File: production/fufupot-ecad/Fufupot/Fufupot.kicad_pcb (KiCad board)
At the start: 4 copper layers, 127 x 127 mm, 56 parts, among them IC1 FOD3150, J1 Conn_01x04, J10 Conn_01x03, J11 Conn_01x03, J12 Conn_01x02, J2 USB_B, J3 Conn_01x03, J4 Conn_01x02, J5 Conn_01x02, J6 Conn_01x02, J7 Conn_01x02, J8 Conn_01x04, J9 Conn_01x02, SW1 SW_Push, SW2 SW_Push, U1 USBLC6-2SC6, U2 LM5165DRC, U3 FT232RL, U4 ATMEGA328P-PN, U5 STGP8NC60KD

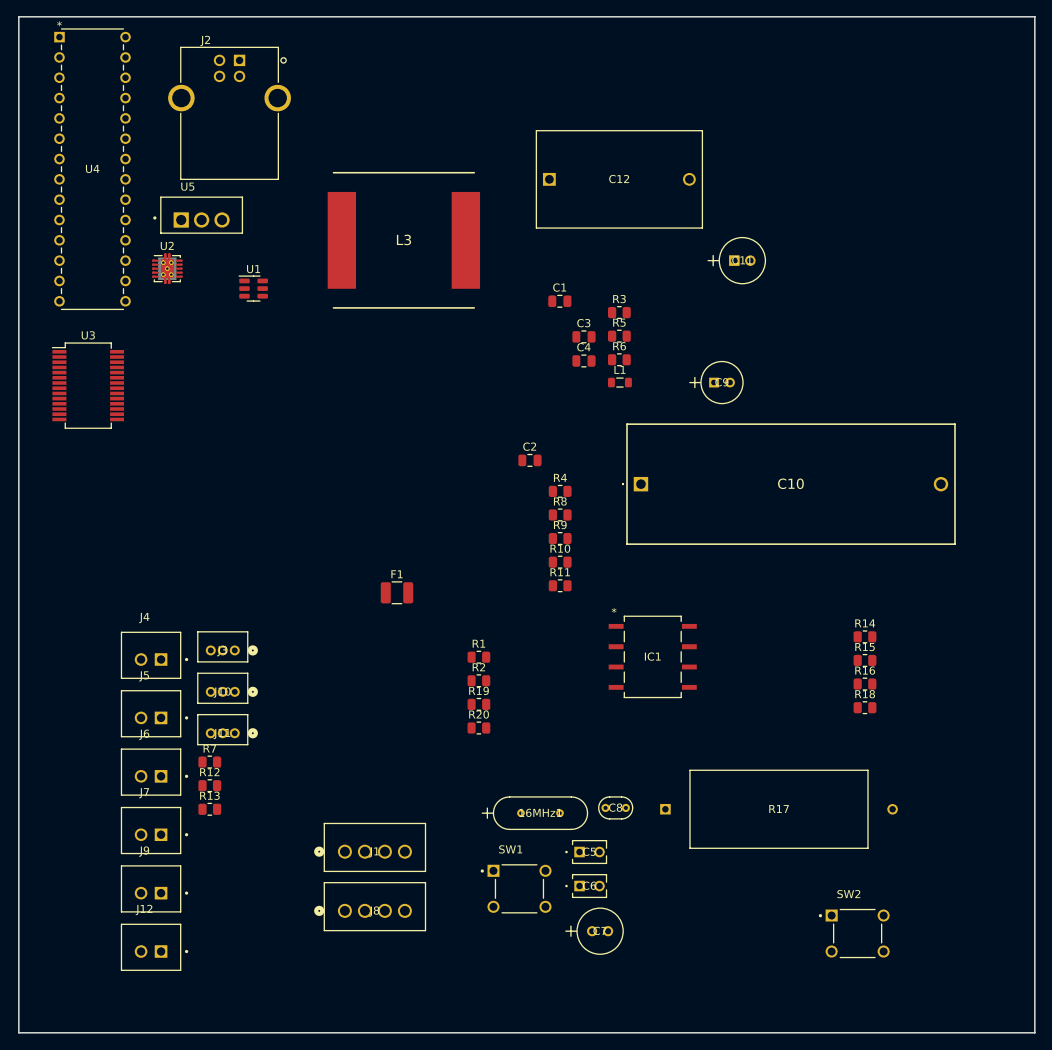
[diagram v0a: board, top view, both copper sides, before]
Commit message: pcb layout
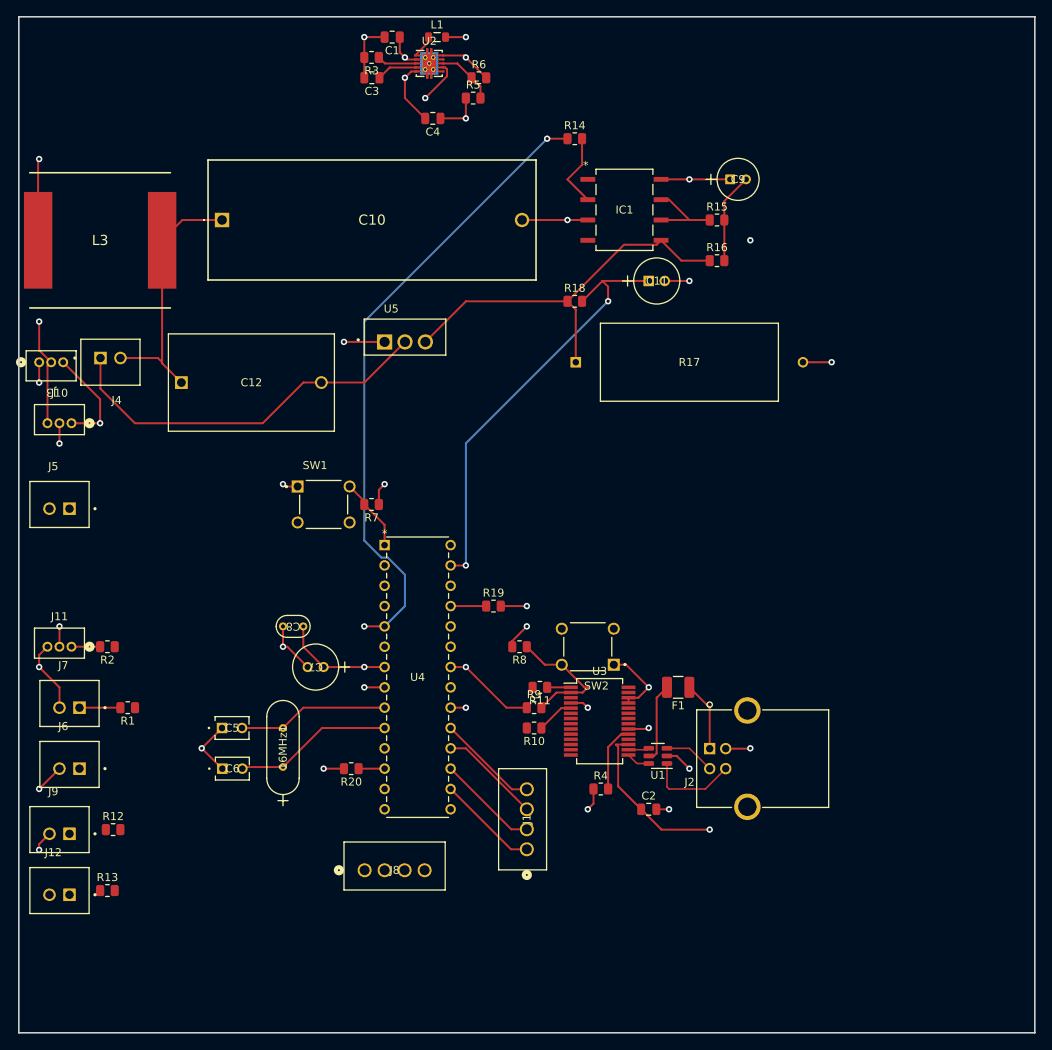
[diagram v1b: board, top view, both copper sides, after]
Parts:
- moved J2 104.2 mm to (132.1, 129.6), turned to 90 degrees
- moved U1 77.2 mm to (125.6, 130.5), turned to 180 degrees
- moved U3 76.5 mm to (118.3, 126.1)
- moved U4 75.4 mm to (91.4, 104.1)
- moved R14 72.1 mm to (115.2, 53.3)
- moved R18 62.4 mm to (115.2, 73.7)
- moved C10 61.9 mm to (71.1, 63.5)
- moved R15 58.1 mm to (133.0, 63.5)
- moved R17 57.0 mm to (115.3, 81.3)
- moved R16 56.1 mm to (133.0, 68.6)
- moved IC1 56.0 mm to (121.4, 62.2)
- moved SW1 53.9 mm to (83.8, 99.1)
- moved C12 52.5 mm to (66.0, 83.8)
- moved SW2 49.2 mm to (116.8, 116.8), turned to 180 degrees
- moved L1 48.9 mm to (98.0, 40.6)
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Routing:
- net GND: track 0.00 -> 116.1 mm, vias 0 -> 20
- net D9: track 0.00 -> 79.1 mm, vias 0 -> 2
- net Net-(IC1-VSS): track 0.00 -> 66.3 mm, vias 0 -> 2
- net A1: track 0.00 -> 54.5 mm, vias 0 -> 2
- net Net-(J4-Pin_1): track 0.00 -> 47.9 mm
- net +5V: track 0.00 -> 33.6 mm, vias 0 -> 9
- net +48V: track 0.00 -> 33.5 mm, vias 0 -> 4
- net Net-(J4-Pin_2): track 0.00 -> 32.7 mm
- net +3V3: track 0.00 -> 20.6 mm, vias 0 -> 1
- net Net-(U4-PB7): track 0.00 -> 19.9 mm
- net Net-(U4-PB6): track 0.00 -> 18.9 mm
- net DTR: track 0.00 -> 16.6 mm
- net SCK: track 0.00 -> 12.7 mm
- net MISO: track 0.00 -> 12.7 mm
- net MOSI: track 0.00 -> 12.7 mm
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- added copper zone on In2.Cu, net +16V
- added copper zone on In2.Cu, net +48V
- added copper zone on In2.Cu, net +5V
